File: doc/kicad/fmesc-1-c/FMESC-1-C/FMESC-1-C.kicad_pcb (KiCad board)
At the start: 2 copper layers, 48 x 48 mm, 118 parts, among them Q1 AON6504, Q10 AON6504, Q11 AON6504, Q12 AON6504, Q13 AON6504, Q14 AON6504, Q15 AON6504, Q16 AON6504, Q17 AON6504, Q18 AON6504, Q19 AON6504, Q2 AON6504, Q20 AON6504, Q21 AON6504, Q22 AON6504, Q23 AON6504, Q24 AON6504, Q3 AON6504, Q4 AON6504, Q5 AON6504, Q6 AON6504, Q7 AON6504, Q8 AON6504, Q9 AON6504, U1 FD6288Q, U2 FD6288Q, U3 FD6288Q, U4 FD6288Q

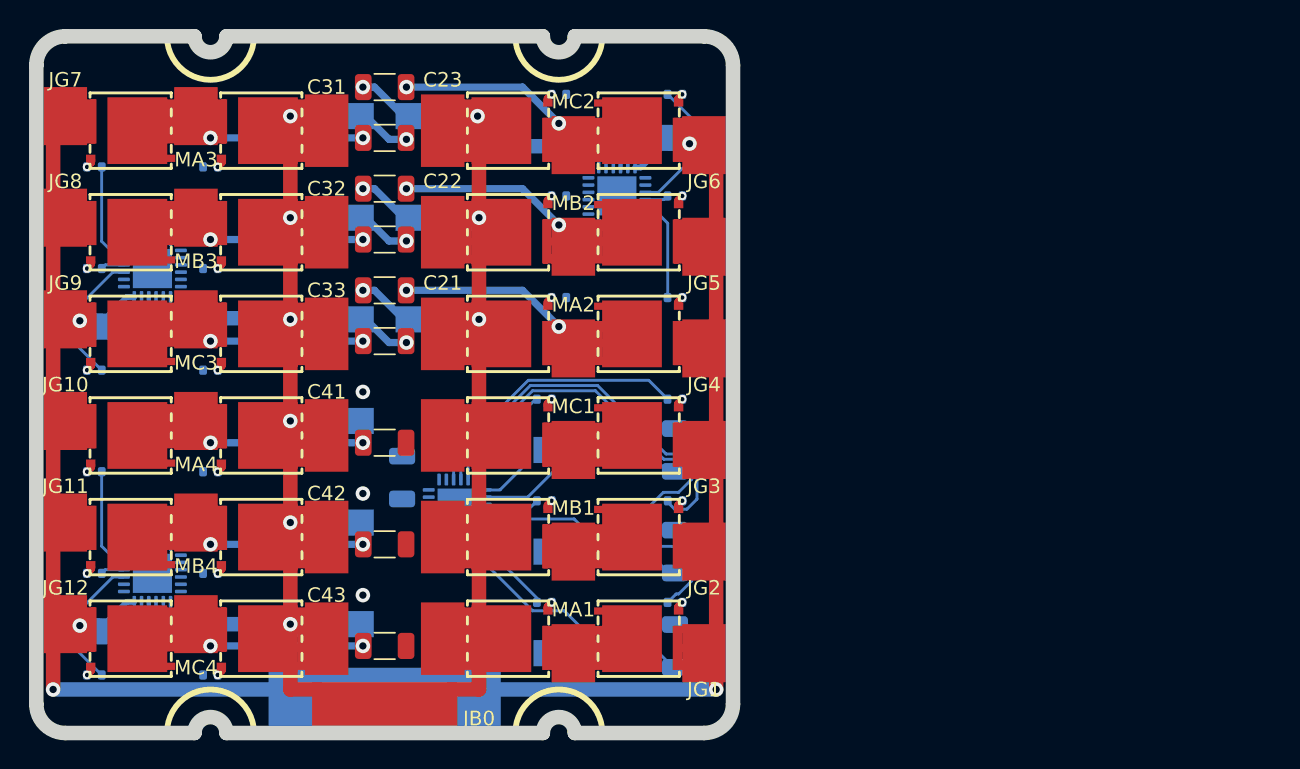
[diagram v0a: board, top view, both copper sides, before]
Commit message: doc/kicad: FMESC-1-C add PCB
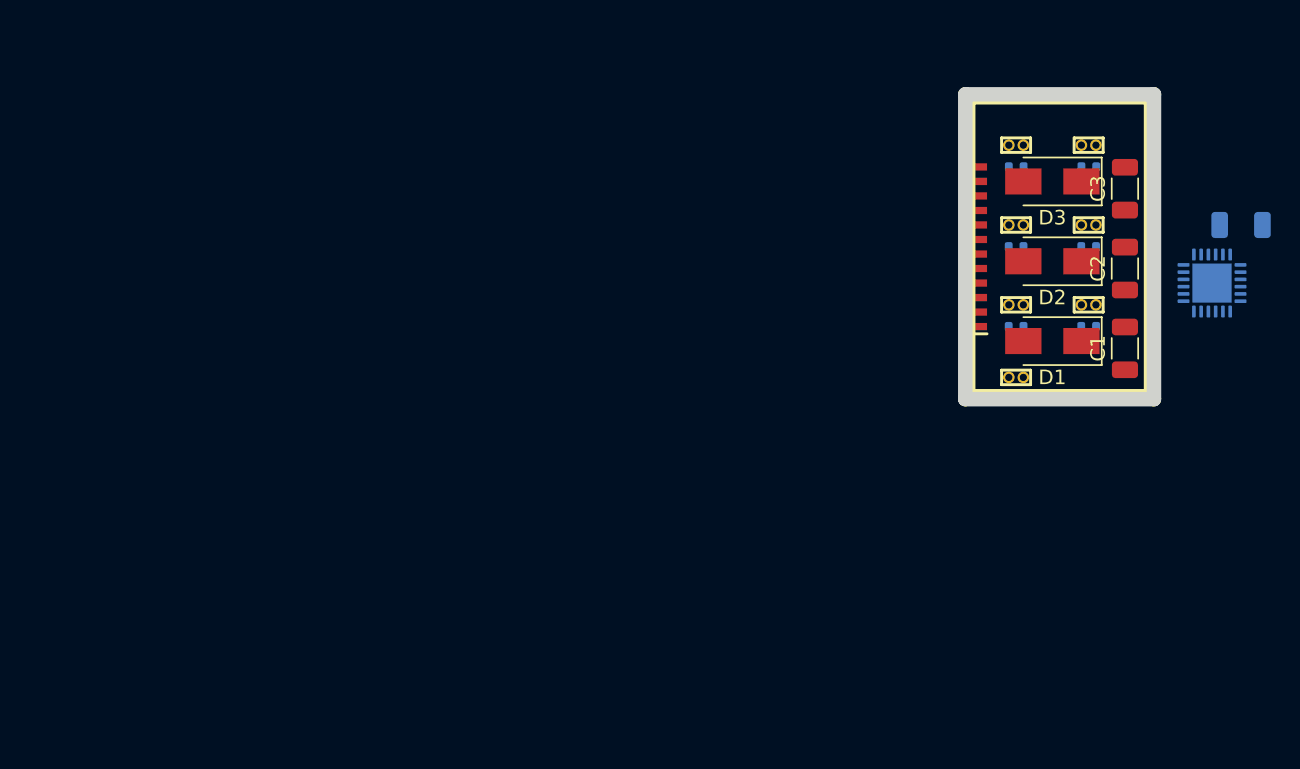
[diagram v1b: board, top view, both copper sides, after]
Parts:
- removed C10, C11, C12, C13, C20, C21, C22, C23, C30, C31, C32, C33, C40, C41, C42, C43: 10u, Capacitor_SMD:C_1206_3216Metric
- removed D11, D12, D13, D21, D22, D23, D31, D32, D33, D41, D42, D43: D, Diode_SMD:D_SMA
- removed JB0: Conn_01x01, fmlibf:JS3x10mm
- removed JB1, JB10, JB11, JB12, JB2, JB3, JB4, JB5, JB6, JB7, JB8, JB9: Conn_01x01, fmlibf:JS3x5mm
- removed JG0: Conn_01x01, fmlibf:JS4x16mm
- removed JG1, JG10, JG11, JG12, JG2, JG3, JG4, JG5, JG6, JG7, JG8, JG9, MA1, MA2, MA3, MA4, MB1, MB2, MB3, MB4, MC1, MC2, MC3, MC4: Conn_01x01, fmlibf:JS3x4mm
- removed Q1, Q10, Q11, Q12, Q13, Q14, Q15, Q16, Q17, Q18, Q19, Q2, Q20, Q21, Q22, Q23, Q24, Q3, Q4, Q5, Q6, Q7, Q8, Q9: AON6504, fmlibf:DFN5x6_8L_EP1_P
- removed R11, R12, R13, R14, R15, R16, R21, R22, R23, R24, R25, R26, R31, R32, R33, R34, R35, R36, R41, R42, R43, R44, R45, R46: 10, Resistor_SMD:R_0402_1005Metric
- removed U2, U3, U4: FD6288Q, Package_DFN_QFN:QFN-24-1EP_4x4mm_P0.5mm_EP2.7x2.7mm
- added C0: 10u, Capacitor_SMD:C_1206_3216Metric, B.Cu at (133.0, 63.0)
- added C1: 10u, Capacitor_SMD:C_1206_3216Metric, F.Cu at (125.0, 71.5)
- added C2: 10u, Capacitor_SMD:C_1206_3216Metric, F.Cu at (125.0, 66.0)
- added C3: 10u, Capacitor_SMD:C_1206_3216Metric, F.Cu at (125.0, 60.5)
- added D1: D, Diode_SMD:D_SMA, F.Cu at (120.0, 71.0)
- added D2: D, Diode_SMD:D_SMA, F.Cu at (120.0, 65.5)
- added D3: D, Diode_SMD:D_SMA, F.Cu at (120.0, 60.0)
- added J1: Conn_01x02, fmlibf:JT_2P_1.0mm, F.Cu at (122.5, 68.5)
- added J2: Conn_01x02, fmlibf:JT_2P_1.0mm, F.Cu at (117.5, 68.5)
- added J3: Conn_01x02, fmlibf:JT_2P_1.0mm, F.Cu at (122.5, 63.0)
- added J4: Conn_01x02, fmlibf:JT_2P_1.0mm, F.Cu at (117.5, 63.0)
- added J5: Conn_01x02, fmlibf:JT_2P_1.0mm, F.Cu at (122.5, 57.5)
- added J6: Conn_01x02, fmlibf:JT_2P_1.0mm, F.Cu at (117.5, 57.5)
- added JC1: Conn_01x12, fmlibf:JS_12P_1.0mm, F.Cu at (115.0, 64.5)
- added JP1: Conn_01x02, fmlibf:JT_2P_1.0mm, F.Cu at (117.5, 73.5)
- added R1: 10, Resistor_SMD:R_0402_1005Metric, B.Cu at (122.5, 70.0)
- added R2: 10, Resistor_SMD:R_0402_1005Metric, B.Cu at (117.5, 70.0)
- added R3: 10, Resistor_SMD:R_0402_1005Metric, B.Cu at (122.5, 64.5)
- added R4: 10, Resistor_SMD:R_0402_1005Metric, B.Cu at (117.5, 64.5)
- added R5: 10, Resistor_SMD:R_0402_1005Metric, B.Cu at (122.5, 59.0)
- added R6: 10, Resistor_SMD:R_0402_1005Metric, B.Cu at (117.5, 59.0)
- moved U1 54.3 mm to (131.0, 67.0), turned to 270 degrees
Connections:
- U1 pad 1: /M1/CAL1 -> /CAL1
- U1 pad 10: /M1/BLG -> /BLG
- U1 pad 11: /M1/ALG -> /ALG
- U1 pad 12: /M1/C1 -> /C1
- U1 pad 13: /M1/CHG -> /CHG
- U1 pad 15: /M1/B1 -> /B1
- U1 pad 16: /M1/BHG -> /BHG
- U1 pad 18: /M1/A1 -> /A1
- U1 pad 19: /M1/AHG -> /AHG
- U1 pad 2: /M1/CBL1 -> /CBL1
- U1 pad 22: /M1/CAH1 -> /CAH1
- U1 pad 23: /M1/CBH1 -> /CBH1
- U1 pad 24: /M1/CCH1 -> /CCH1
- U1 pad 3: /M1/CCL1 -> /CCL1
- U1 pad 9: /M1/CLG -> /CLG
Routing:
- net +BATT: track 256.5 -> 0.00 mm, vias 9 -> 0
- net GND: track 171.0 -> 0.00 mm, vias 5 -> 0
- net /M1/ALG: track 35.5 -> 0.00 mm
- net /M1/BLG: track 27.2 -> 0.00 mm
- net /M2/C1: track 23.8 -> 0.00 mm, vias 2 -> 0
- net /M2/A1: track 23.8 -> 0.00 mm, vias 2 -> 0
- net /M2/B1: track 23.5 -> 0.00 mm, vias 2 -> 0
- net /M4/B1: track 23.3 -> 0.00 mm, vias 2 -> 0
- net /M3/C1: track 23.2 -> 0.00 mm, vias 2 -> 0
- net /M4/C1: track 23.1 -> 0.00 mm, vias 2 -> 0
- net /M4/A1: track 23.0 -> 0.00 mm, vias 2 -> 0
- net /M3/B1: track 23.0 -> 0.00 mm, vias 2 -> 0
- net /M3/A1: track 23.0 -> 0.00 mm, vias 2 -> 0
- net /M1/CLG: track 19.1 -> 0.00 mm
- net Net-(C1-Pad1): track 17.4 -> 0.00 mm, vias 1 -> 0
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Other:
- board size 48 x 48 mm -> 13 x 21 mm

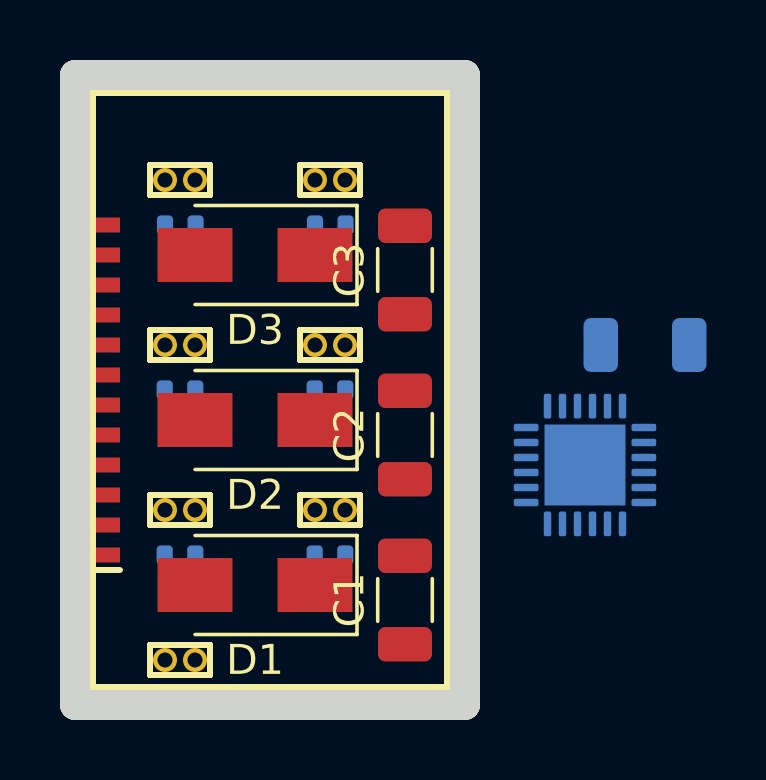
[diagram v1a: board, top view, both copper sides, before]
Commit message: doc/kicad: FMESC-1-C PCB layout
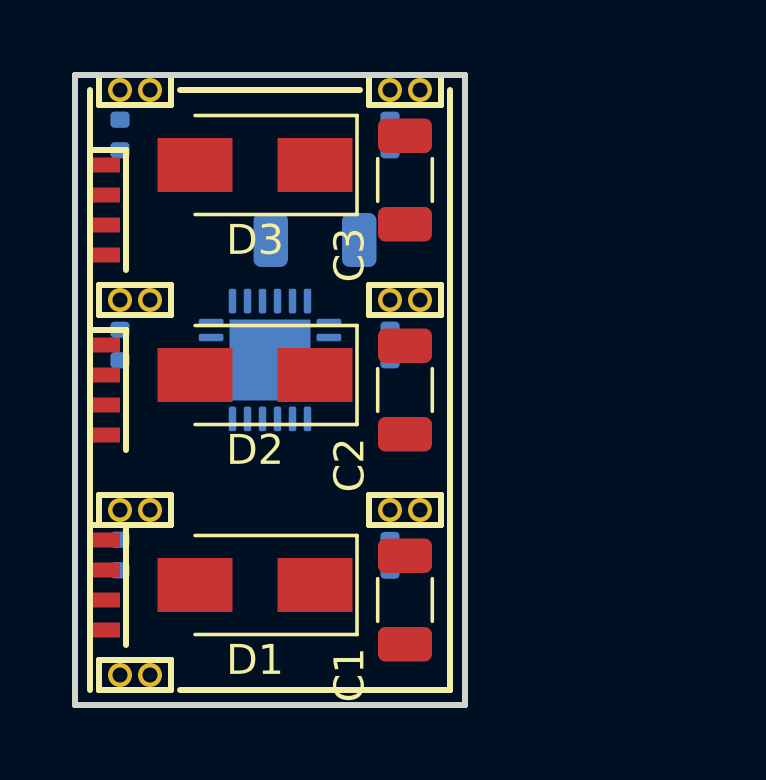
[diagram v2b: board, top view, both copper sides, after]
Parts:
- added JC2: Conn_01x04, fmlibf:JS_4P_1.0mm, F.Cu at (115.0, 64.5)
- added JC3: Conn_01x04, fmlibf:JS_4P_1.0mm, F.Cu at (115.0, 71.0)
- JC1: value Conn_01x12 -> Conn_01x04; footprint fmlibf:JS_12P_1.0mm -> fmlibf:JS_4P_1.0mm
- moved C0 11.5 mm to (122.0, 59.5)
- moved U1 11.1 mm to (120.5, 63.5)
- moved JC1 6.00 mm to (115.0, 58.5), turned to 270 degrees
- moved J5 3.91 mm to (125.0, 54.5), turned to 180 degrees
- moved R6 3.61 mm to (115.5, 56.0), turned to 90 degrees
- moved R5 3.60 mm to (124.5, 56.0), turned to 90 degrees
- moved J6 3.35 mm to (116.0, 54.5), turned to 180 degrees
- moved C3 3.00 mm to (125.0, 57.5)
- moved D3 3.00 mm to (120.0, 57.0)
- moved J3 2.92 mm to (125.0, 61.5), turned to 180 degrees
- moved J1 2.50 mm to (125.0, 68.5), turned to 180 degrees
- moved R3 2.50 mm to (124.5, 63.0), turned to 90 degrees
- moved R4 2.50 mm to (115.5, 63.0), turned to 90 degrees
- moved J4 2.12 mm to (116.0, 61.5), turned to 180 degrees
- moved R1 2.00 mm to (124.5, 70.0), turned to 90 degrees
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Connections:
- JC1 pad 1: /CAL1 -> GND
- JC1 pad 2: /CBL1 -> /CAL1
- JC1 pad 3: /CCL1 -> /CBL1
- JC1 pad 4: /CAH1 -> /CCL1
